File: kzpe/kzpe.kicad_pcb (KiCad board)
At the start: 2 copper layers, 32 x 22 mm, 22 parts, among them J1 Conn_12VIN, J2 Conn_FAN, J3 Conn_NTC, Q1 IRLL014TRPBF-BE3, U1 LM555xM, U2 TL081, U3 LF50ABDT-TR

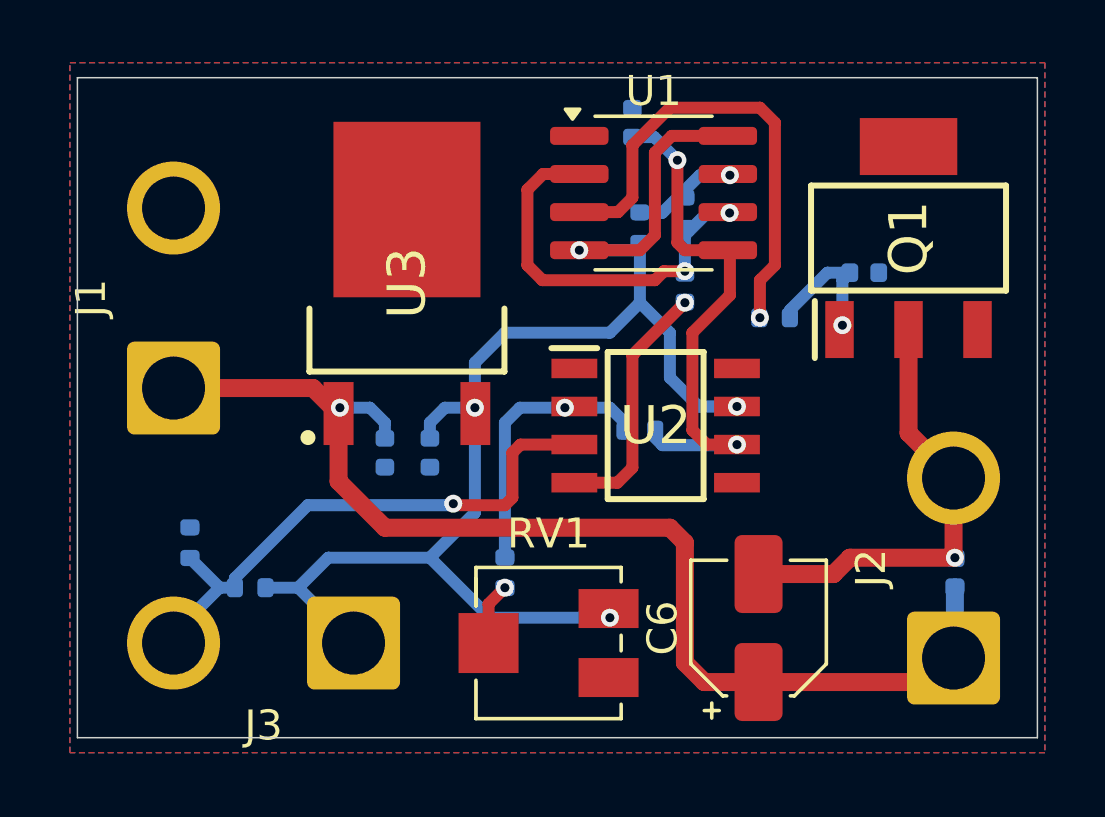
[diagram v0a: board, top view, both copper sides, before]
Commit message: 0912
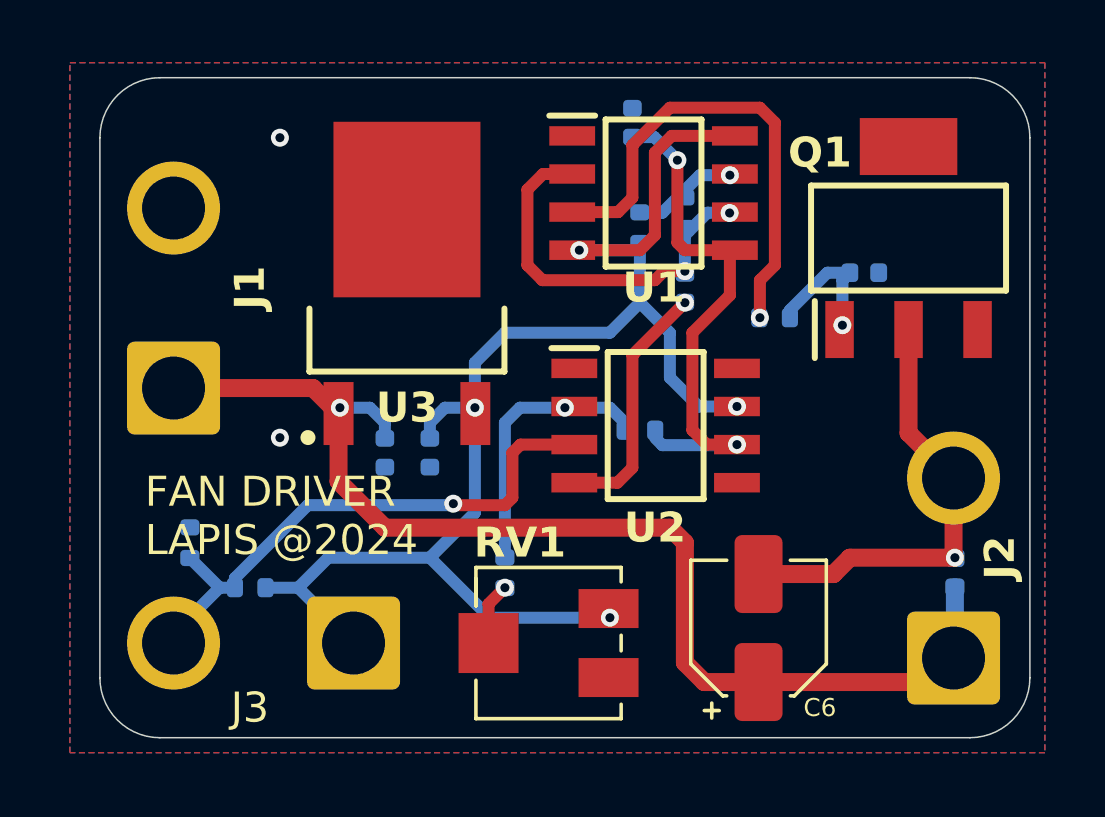
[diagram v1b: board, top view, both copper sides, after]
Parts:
- U1: footprint Package_SO:SOIC-8_3.9x4.9mm_P1.27mm -> kzpe_fp:SOIC127P600X175-8N
- U2: footprint Library:TL081 -> kzpe_fp:SOIC127P600X175-8N
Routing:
- net GND: vias 1 -> 3
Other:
- board size 32 x 22 mm -> 31 x 22 mm
- board text added: "FAN DRIVER LAPIS @2024"

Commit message: 1012
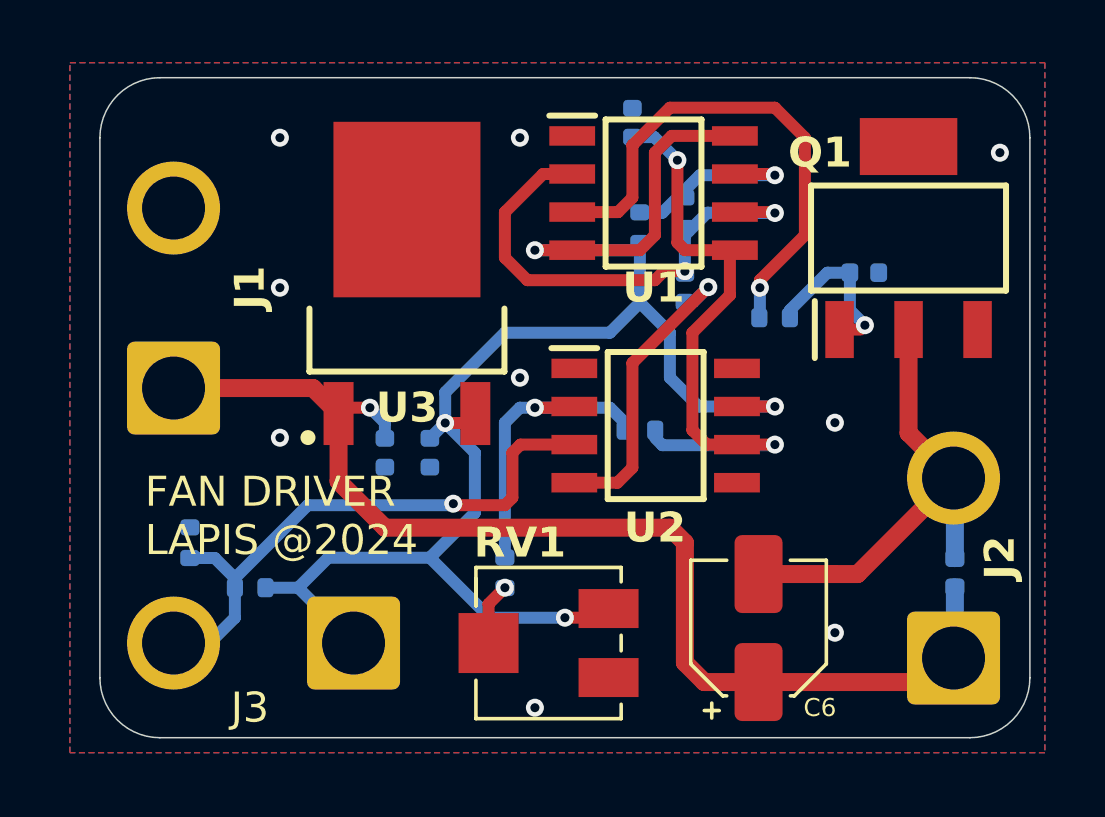
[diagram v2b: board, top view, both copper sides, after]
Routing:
- net +5V: track 48.8 -> 54.8 mm
- net Net-(U1-THR): track 13.1 -> 18.3 mm
- net Net-(U1-DIS): track 3.76 -> 6.61 mm
- net Net-(U1-CV): track 17.4 -> 19.9 mm
- net GND: track 8.39 -> 10.2 mm, vias 3 -> 10
- net Net-(U2--): track 9.15 -> 10.5 mm
- net Net-(Q1-G): track 4.62 -> 5.83 mm
- net Net-(U1-Q): track 15.9 -> 17.0 mm
- net Net-(J3-Pin_2): track 18.8 -> 19.9 mm
- net Net-(D1-A): track 15.0 -> 16.1 mm, vias 1 -> 0

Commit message: 1112
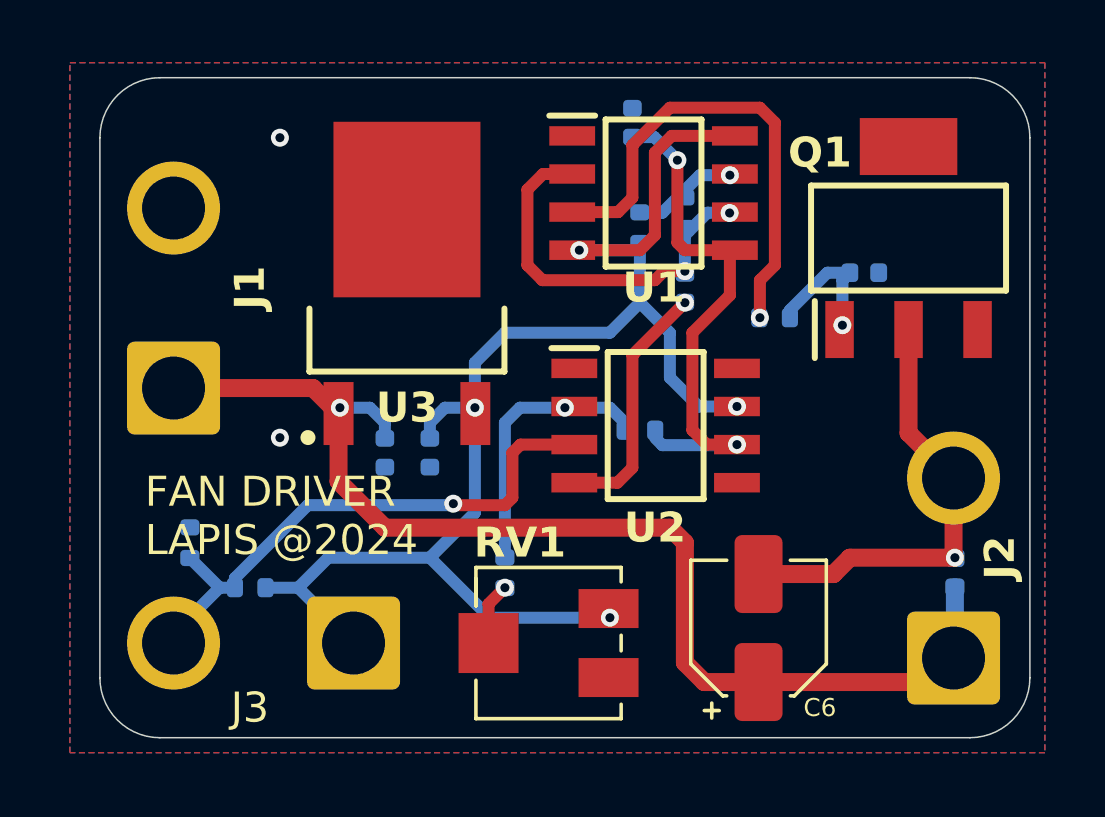
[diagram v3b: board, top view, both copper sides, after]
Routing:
- net +5V: track 54.8 -> 48.8 mm
- net Net-(U1-THR): track 18.3 -> 13.1 mm
- net Net-(U1-DIS): track 6.61 -> 3.76 mm
- net Net-(U1-CV): track 19.9 -> 17.4 mm
- net GND: track 10.2 -> 8.39 mm, vias 10 -> 3
- net Net-(U2--): track 10.5 -> 9.15 mm
- net Net-(Q1-G): track 5.83 -> 4.62 mm
- net Net-(U1-Q): track 17.0 -> 15.9 mm
- net Net-(J3-Pin_2): track 19.9 -> 18.8 mm
- net Net-(D1-A): track 16.1 -> 15.0 mm, vias 0 -> 1
